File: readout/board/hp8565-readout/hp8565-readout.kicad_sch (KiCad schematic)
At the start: 18 parts, among them J1 Pin_Header, J2 Pin_Header, J3 DIP Socket, J4 Pin_Header, J5 Masach_MS230-20S, P1 DIP Pins, U1 ATmega4809-M, U2 GD75232DB

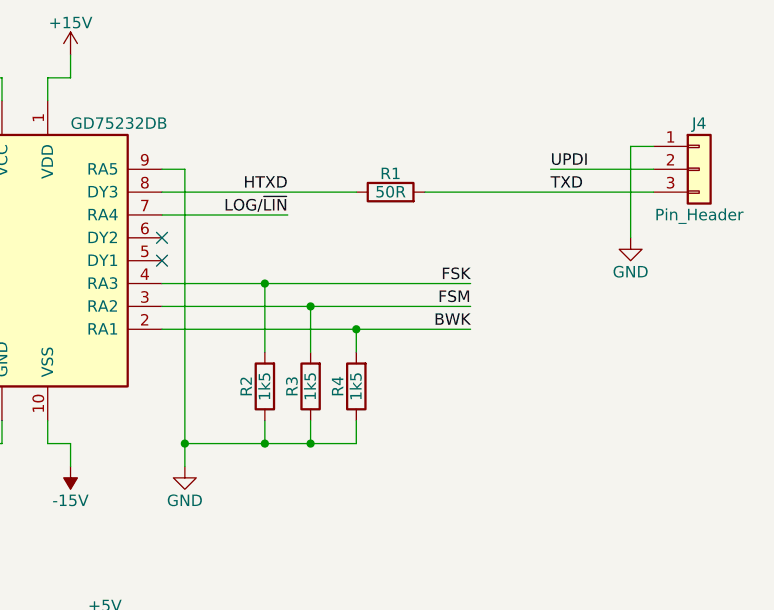
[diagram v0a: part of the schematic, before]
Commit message: Clean up silkscreen and stuff.
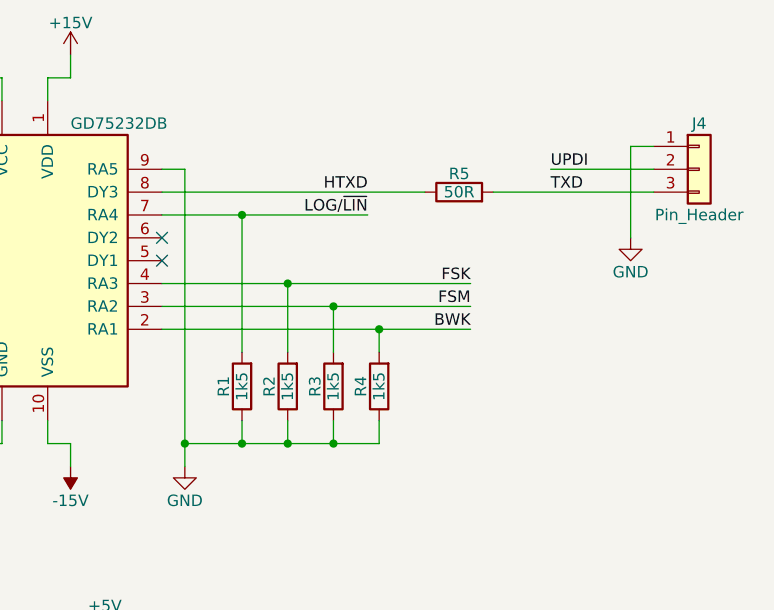
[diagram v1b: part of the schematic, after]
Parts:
- added R1: 1k5, Resistor_SMD:R_0402_1005Metric, symbol Device:R
- renumbered R1 to R5
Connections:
- net GND: now also R1.1
- net LOG/~{LIN}: now also R1.2
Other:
- moved on the sheet: R2, R3, R4, R5
